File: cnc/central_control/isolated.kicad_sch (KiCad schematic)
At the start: 25 parts, among them U10 PC817, U14 PC817, U15 PC817, U16 PC817, U17 PC817, U18 PC817, U19 PC817, U5 PC817, U6 PC817, U7 PC817, U8 PC817, U9 PC817

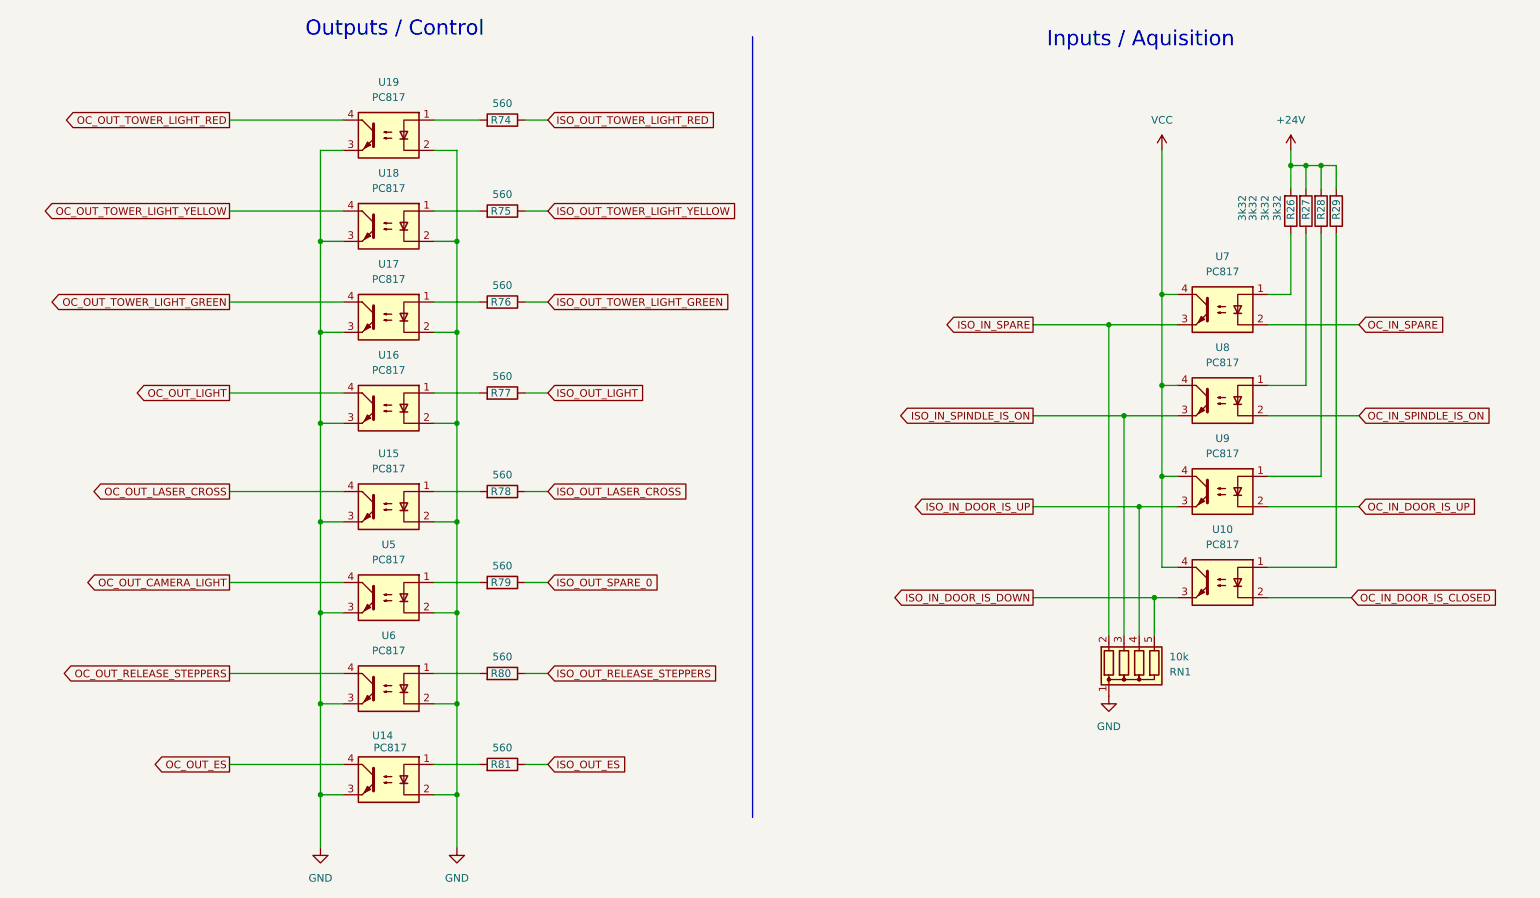
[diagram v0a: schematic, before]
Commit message: Sent to production
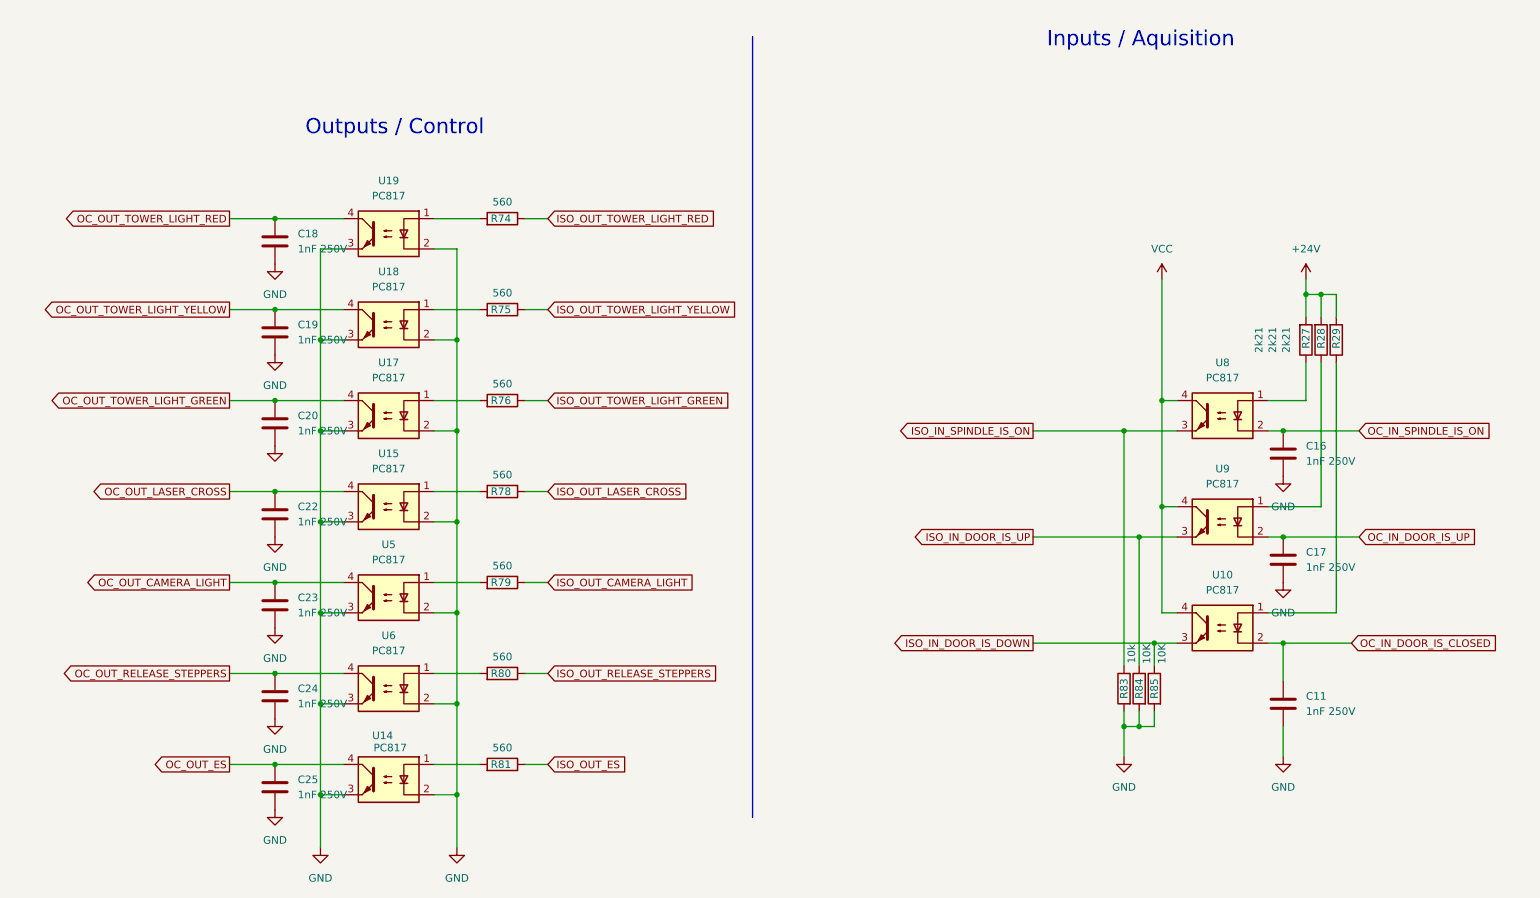
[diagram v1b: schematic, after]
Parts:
- removed R26: 3k32, Resistor_SMD:R_1206_3216Metric_Pad1.30x1.75mm_HandSolder, symbol Device:R
- removed R77: 560, Resistor_SMD:R_1206_3216Metric_Pad1.30x1.75mm_HandSolder, symbol Device:R
- removed RN1: 10k, Resistor_THT:R_Array_SIP5, symbol Device:R_Network04
- removed U16, U7: PC817, Package_DIP:DIP-4_W7.62mm, symbol Isolator:PC817
- added C11, C16, C17, C18, C19, C20, C22, C23, C24, C25: 1nF 250V, Capacitor_SMD:C_1206_3216Metric_Pad1.33x1.80mm_HandSolder, symbol Device:C
- added R83: 10k, Resistor_SMD:R_1206_3216Metric_Pad1.30x1.75mm_HandSolder, symbol Device:R
- added R84, R85: 10K, Resistor_SMD:R_1206_3216Metric_Pad1.30x1.75mm_HandSolder, symbol Device:R
- R27, R28, R29: value 3k32 -> 2k21
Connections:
- net GND: now also C11.2, C16.2, C17.2, C18.2, C19.2, C20.2, C22.2, C23.2, C24.2, C25.2, R83.2, R84.2, R85.2
- net ISO_IN_DOOR_IS_DOWN: now also R85.1
- net ISO_IN_DOOR_IS_UP: now also R84.1
- net ISO_IN_SPINDLE_IS_ON: now also R83.1
- net OC_IN_DOOR_IS_CLOSED: now also C11.1
- net OC_IN_DOOR_IS_UP: now also C17.1
- net OC_IN_SPINDLE_IS_ON: now also C16.1
- net OC_OUT_CAMERA_LIGHT: now also C23.1
- net OC_OUT_ES: now also C25.1
- net OC_OUT_LASER_CROSS: now also C22.1
- net OC_OUT_RELEASE_STEPPERS: now also C24.1
- net OC_OUT_TOWER_LIGHT_GREEN: now also C20.1
- net OC_OUT_TOWER_LIGHT_RED: now also C18.1
- net OC_OUT_TOWER_LIGHT_YELLOW: now also C19.1
- net ISO_OUT_SPARE_0 renamed ISO_OUT_CAMERA_LIGHT
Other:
- moved on the sheet: R27, R28, R29, R74, R75, R76, U10, U17, U18, U19, U8, U9
